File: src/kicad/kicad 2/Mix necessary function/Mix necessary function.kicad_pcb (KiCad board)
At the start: 2 copper layers, 53 x 58 mm, 22 parts, among them SW1 02-JST, SW2 02-JST

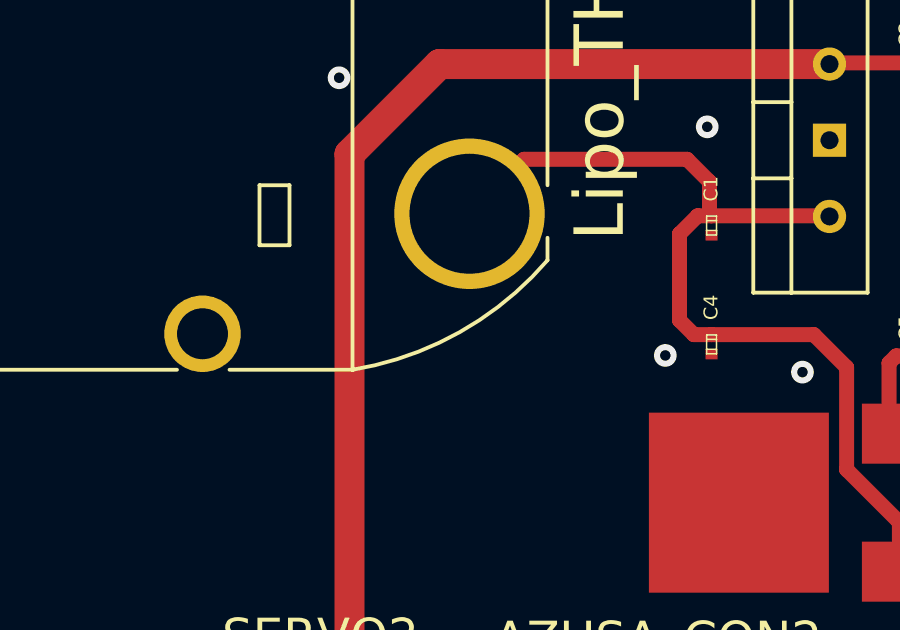
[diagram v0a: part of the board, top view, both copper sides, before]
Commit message: twelite
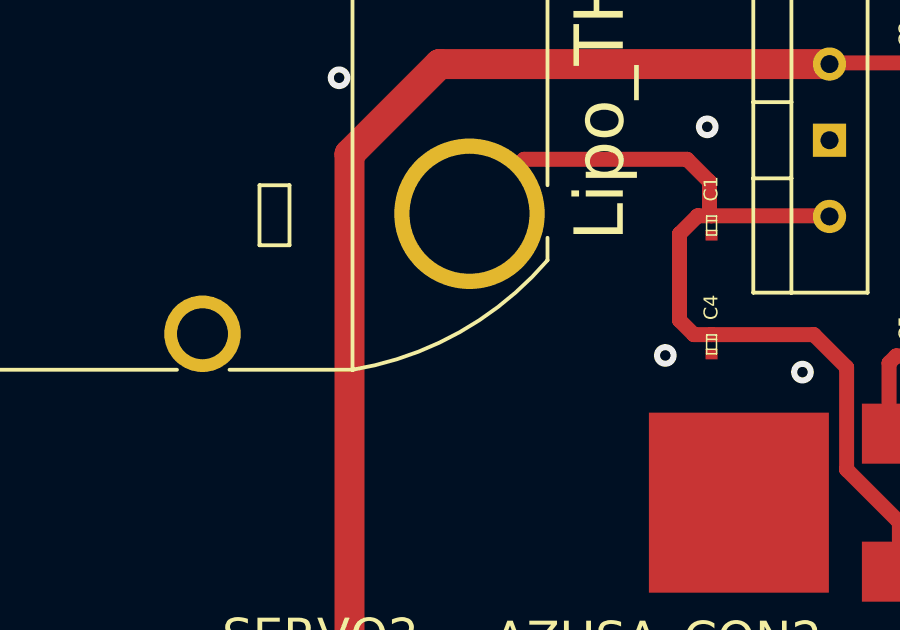
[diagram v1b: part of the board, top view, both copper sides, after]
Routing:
- net N$9: vias 1 -> 0
- net N$8: vias 1 -> 0
- net N$7: vias 1 -> 0
- net N$6: vias 1 -> 0
- net N$5: vias 1 -> 0
- net N$4: vias 1 -> 0
- net N$3: vias 1 -> 0
- net N$18: vias 1 -> 0
- net N$17: vias 1 -> 0
- net N$16: vias 1 -> 0
- net N$15: vias 1 -> 0
- net N$14: vias 1 -> 0
- net N$12: vias 1 -> 0
- net N$11: vias 1 -> 0
- net N$10: vias 1 -> 0
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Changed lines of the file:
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@@
       (outputformat 1)
       (mirror false)
-      (drillshape 1)
+      (drillshape 0)
       (scaleselection 1)
-      (outputdirectory "")
+      (outputdirectory "gerber/")
     )
   )
@@
   (net 9 "PWM2_SERVO")
   (net 10 "PWM1_SERVO")
-  (net 11 "N$1")
-  (net 12 "N$3")
-  (net 13 "N$4")
-  (net 14 "N$5")
-  (net 15 "N$6")
-  (net 16 "N$7")
-  (net 17 "N$8")
-  (net 18 "N$9")
-  (net 19 "N$10")
-  (net 20 "N$11")
-  (net 21 "N$12")
-  (net 22 "N$13")
-  (net 23 "N$14")
-  (net 24 "N$15")
-  (net 25 "N$16")
-  (net 26 "N$17")
-  (net 27 "N$18")
+  (net 11 "N$13")
   (footprint "Mix necessary function:ＮＪＭ７８０６ＦＡ-6V" (layer "F.Cu")
     (at 155.0011 100.0036 90)
@@
     (fp_line (start 10.65 -8) (end 10.65 -3.9)
       (stroke (width 0.127) (type solid)) (layer "F.SilkS"))
-    (fp_arc (start -7 2.6) (mid -9.398063 -0.328203) (end -10.65 -3.9)
+    (fp_arc (start -7 2.6) (mid -9.398061 -0.328204) (end -10.65 -3.9)
       (stroke (width 0.127) (type solid)) (layer "F.SilkS"))
     (fp_arc (start 10.65 -3.9) (mid 9.398063 -0.328203) (end 7 2.6)
@@
   (segment (start 159.145781 107.1932) (end 160.2911 108.338519) (width 0.5) (layer "F.Cu") (net 1))
   (segment (start 160.4311 120.2936) (end 160.2911 120.1536) (width 0.5) (layer "F.Cu") (net 1))
+  (via (at 137.1141 118.5266) (size 0.7564) (drill 0.35) (layers "F.Cu" "B.Cu") (net 2))
+  (via (at 169.8801 123.7336) (size 0.7564) (drill 0.35) (layers "F.Cu" "B.Cu") (net 2))
+  (via (at 155.9101 87.2216) (size 0.7564) (drill 0.35) (layers "F.Cu" "B.Cu") (net 2))
+  (via (at 144.3361 119.4146) (size 0.7564) (drill 0.35) (layers "F.Cu" "B.Cu") (net 2))
+  (via (at 162.4511 124.6066) (size 0.7564) (drill 0.35) (layers "F.Cu" "B.Cu") (net 2))
+  (via (at 146.9401 131.6406) (size 0.7564) (drill 0.35) (layers "F.Cu" "B.Cu") (free) (net 2))
+  (via (at 154.1001 107.7326) (size 0.7564) (drill 0.35) (layers "F.Cu" "B.Cu") (net 2))
+  (via (at 136.3521 131.9886) (size 0.7564) (drill 0.35) (layers "F.Cu" "B.Cu") (net 2))
+  (via (at 149.5281 107.1766) (size 0.7564) (drill 0.35) (layers "F.Cu" "B.Cu") (net 2))
+  (via (at 136.4791 123.2256) (size 0.7564) (drill 0.35) (layers "F.Cu" "B.Cu") (net 2))
+  (via (at 150.9251 99.5566) (size 0.7564) (drill 0.35) (layers "F.Cu" "B.Cu") (net 2))
+  (via (at 138.6541 97.9206) (size 0.7564) (drill 0.35) (layers "F.Cu" "B.Cu") (net 2))
+  (via (at 167.3401 87.2216) (size 0.7564) (drill 0.35) (layers "F.Cu" "B.Cu") (net 2))
+  (via (at 158.8781 104.1446) (size 0.7564) (drill 0.35) (layers "F.Cu" "B.Cu") (net 2))
+  (via (at 148.0191 123.2246) (size 0.7564) (drill 0.35) (layers "F.Cu" "B.Cu") (net 2))
+  (via (at 163.0221 131.2266) (size 0.7564) (drill 0.35) (layers "F.Cu" "B.Cu") (net 2))
   (segment (start 165.1511 99.5736) (end 165.1511 90.1436) (width 1.016) (layer "F.Cu") (net 3))
   (segment (start 156.503556 88.4752) (end 166.482968 88.4752) (width 1.016) (layer "F.Cu") (net 4))
@@
   (segment (start 135.4611 129.0036) (end 135.4611 129.4636) (width 0.2) (layer "F.Cu") (net 10))
   (segment (start 146.0011 131.0036) (end 147.7471 129.2576) (width 0.2) (layer "F.Cu") (net 10))
-  (via (at 148.0191 123.2246) (size 0.7564) (drill 0.35) (layers "F.Cu" "B.Cu") (net 11))
-  (via (at 146.9401 131.6406) (size 0.7564) (drill 0.35) (layers "F.Cu" "B.Cu") (net 12))
-  (via (at 137.1141 118.5266) (size 0.7564) (drill 0.35) (layers "F.Cu" "B.Cu") (net 13))
-  (via (at 144.3361 119.4146) (size 0.7564) (drill 0.35) (layers "F.Cu" "B.Cu") (net 14))
-  (via (at 136.3521 131.9886) (size 0.7564) (drill 0.35) (layers "F.Cu" "B.Cu") (net 15))
-  (via (at 136.4791 123.2256) (size 0.7564) (drill 0.35) (layers "F.Cu" "B.Cu") (net 16))
-  (via (at 154.1001 107.7326) (size 0.7564) (drill 0.35) (layers "F.Cu" "B.Cu") (net 17))
-  (via (at 149.5281 107.1766) (size 0.7564) (drill 0.35) (layers "F.Cu" "B.Cu") (net 18))
-  (via (at 158.8781 104.1446) (size 0.7564) (drill 0.35) (layers "F.Cu" "B.Cu") (net 19))
-  (via (at 150.9251 99.5566) (size 0.7564) (drill 0.35) (layers "F.Cu" "B.Cu") (net 20))
-  (via (at 138.6541 97.9206) (size 0.7564) (drill 0.35) (layers "F.Cu" "B.Cu") (net 21))
-  (via (at 162.5141 118.9076) (size 0.7564) (drill 0.35) (layers "F.Cu" "B.Cu") (net 22))
-  (via (at 162.4511 124.6066) (size 0.7564) (drill 0.35) (layers "F.Cu" "B.Cu") (net 23))
-  (via (at 169.8801 123.7336) (size 0.7564) (drill 0.35) (layers "F.Cu" "B.Cu") (net 24))
-  (via (at 163.0221 131.2266) (size 0.7564) (drill 0.35) (layers "F.Cu" "B.Cu") (net 25))
-  (via (at 155.9101 87.2216) (size 0.7564) (drill 0.35) (layers "F.Cu" "B.Cu") (net 26))
-  (via (at 167.3401 87.2216) (size 0.7564) (drill 0.35) (layers "F.Cu" "B.Cu") (net 27))
+  (via (at 162.5141 118.9076) (size 0.7564) (drill 0.35) (layers "F.Cu" "B.Cu") (net 11))
   (zone (net 2) (net_name "GND") (layer "F.Cu") (hatch edge 0.5)
     (priority 6)
